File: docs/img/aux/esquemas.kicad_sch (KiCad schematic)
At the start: 60 parts

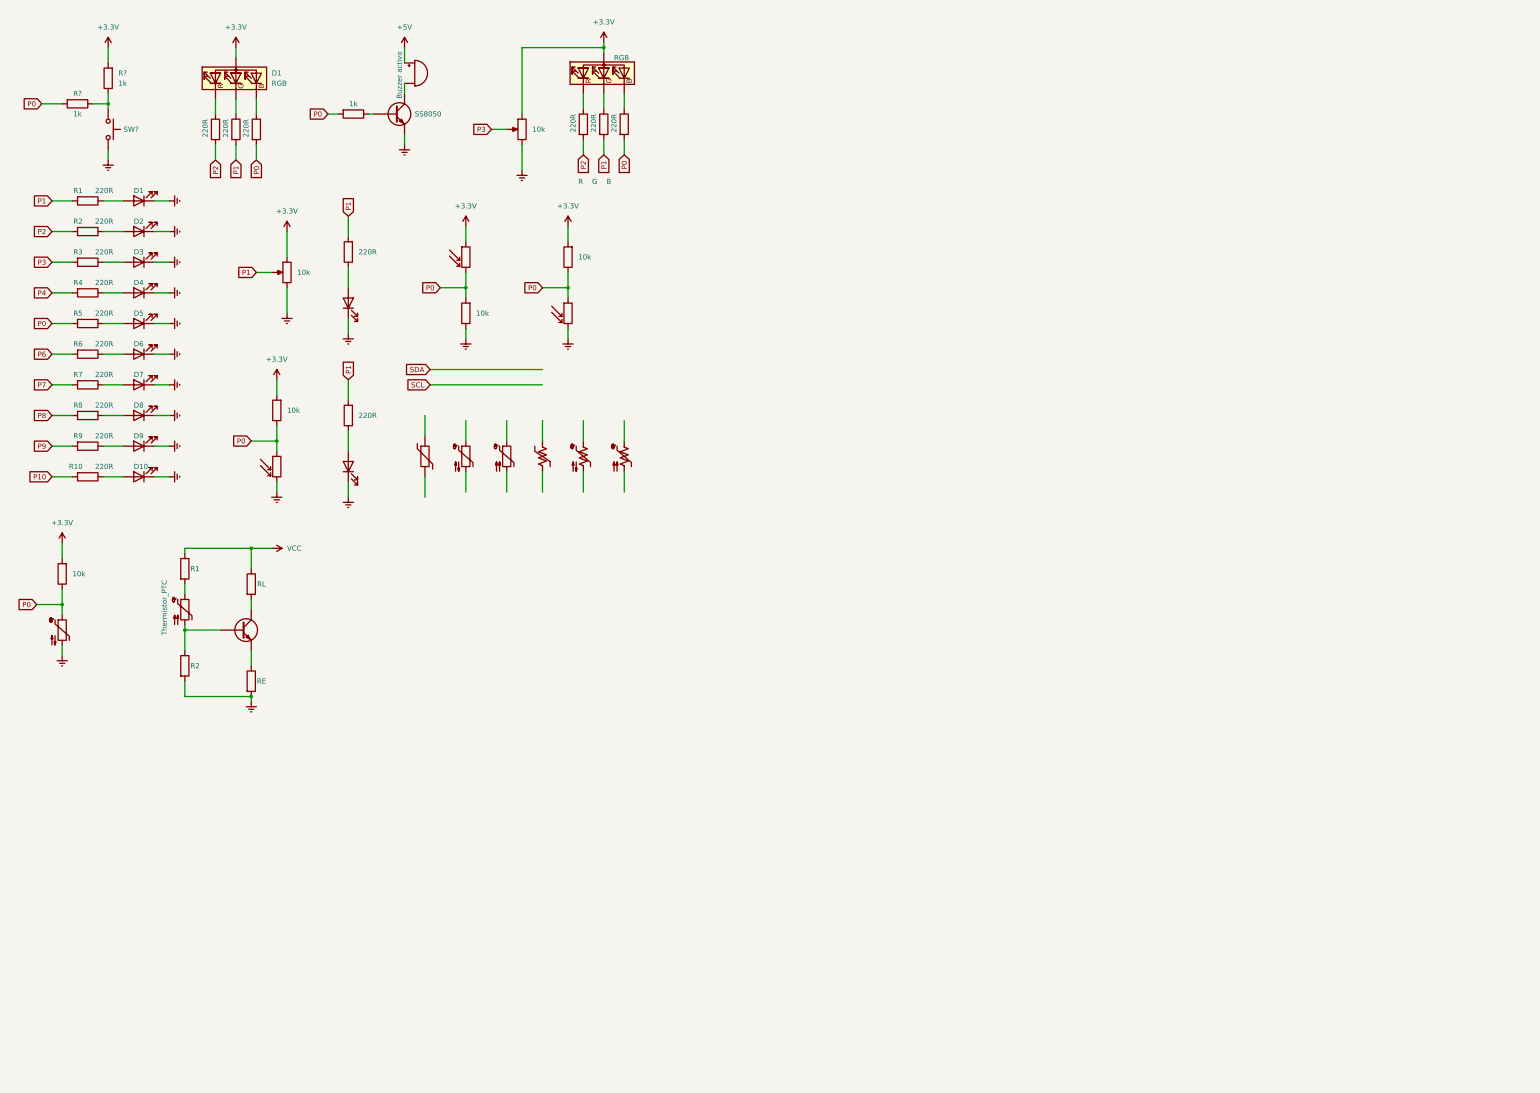
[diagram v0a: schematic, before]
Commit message: actualizar hasta PaP
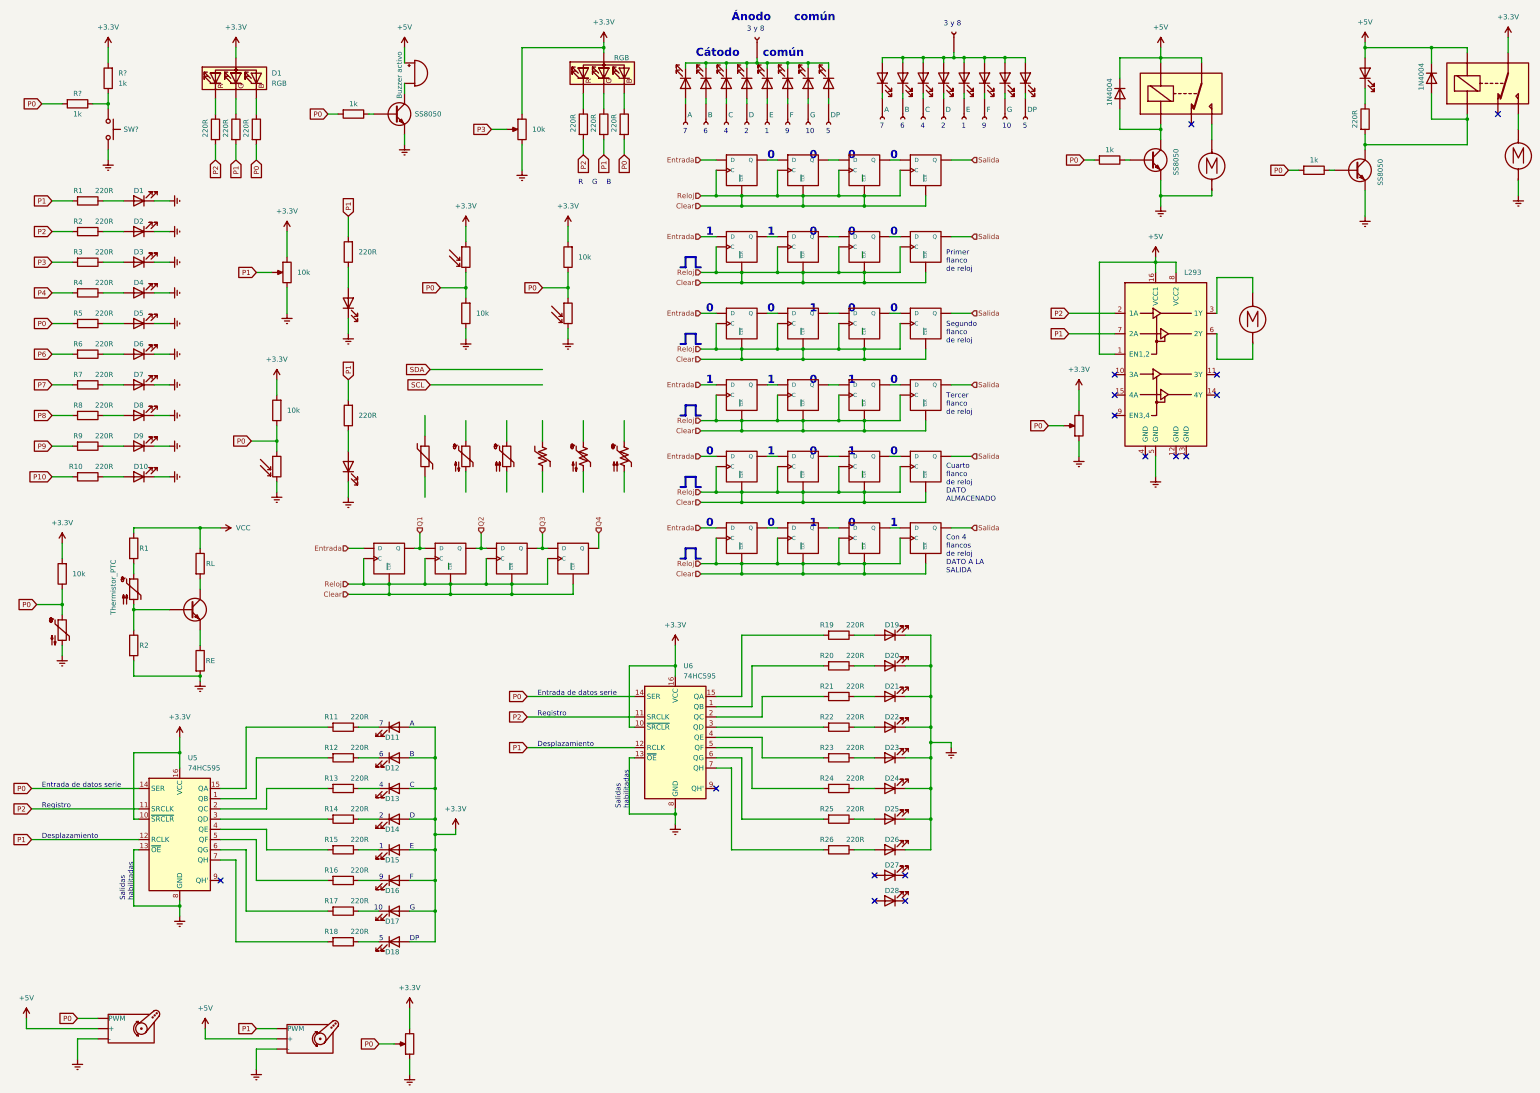
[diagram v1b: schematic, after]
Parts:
- added D11, D12, D13, D14, D15, D16, D17, D18, D19, D20, D21, D22, D23, D24, D25, D26, D27, D28, D? (x17): LED, symbol Device:LED
- added D? (x2): 1N4004, Diode_THT:D_DO-41_SOD81_P10.16mm_Horizontal, symbol Diode:1N4004
- added J? (x2): F, symbol Connector:Conn_01x01_Female
- added J? (x2): C, symbol Connector:Conn_01x01_Female
- added J? (x2): G, symbol Connector:Conn_01x01_Female
- added J? (x2): DP, symbol Connector:Conn_01x01_Female
- added J? (x2): A, symbol Connector:Conn_01x01_Female
- added J? (x2): B, symbol Connector:Conn_01x01_Female
- added J? (x2): D, symbol Connector:Conn_01x01_Female
- added J? (x2): Conn_01x01_Female, symbol Connector:Conn_01x01_Female
- added J? (x2): E, symbol Connector:Conn_01x01_Female
- added K? (x2): FINDER-32.21-x000, Relay_THT:Relay_SPDT_Finder_32.21-x000, symbol Relay:FINDER-32.21-x000
- added M? (x3): Motor_DC, symbol Motor:Motor_DC
- added M? (x2): Motor_Servo, symbol Motor:Motor_Servo
- added Q? (x2): SS8050, Package_TO_SOT_THT:TO-92_Inline, symbol Transistor_BJT:2N3904
- added R11, R12, R13, R14, R15, R16, R17, R18, R19, R20, R21, R22, R23, R24, R25, R26, R?: 220R, symbol Device:R
- added R? (x2): 1k, symbol Device:R
- added RV? (x2): R_Potentiometer, symbol Device:R_Potentiometer
- added U1, U2, U3, U4, U? (x24): 74LVC1G175, symbol 74xGxx:74LVC1G175
- added U5, U6: 74HC595, symbol 74xx:74HC595
- added U?: L293, Package_DIP:DIP-16_W7.62mm, symbol Driver_Motor:L293
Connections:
- net +3.3V: now also D11.2 (A), D12.2 (A), D13.2 (A), D14.2 (A), D15.2 (A), D16.2 (A), D17.2 (A), D18.2 (A), K?.11, RV?.3, RV?.3, U5.10 (~{SRCLR}), U5.16 (VCC), U6.10 (~{SRCLR}), U6.16 (VCC)
- net +5V: now also D?.1 (K), D?.1 (K), D?.2 (A), K?.11, K?.A2, K?.A2, M?.2 (+), M?.2 (+), U?.1 (EN1,2), U?.16 (VCC1), U?.8 (VCC2)
- net GNDREF: now also M?.2 (-), M?.2 (-), Q?.1 (E), Q?.1 (E), RV?.1, RV?.1, U?.5 (GND)
- net P0: now also M?.1 (PWM), R?.2, R?.2, RV?.2, RV?.2, U5.14 (SER), U6.14 (SER)
- net P1: now also M?.1 (PWM), U5.12 (RCLK), U6.12 (RCLK), U?.7 (2A)
- net P2: now also U5.11 (SRCLK), U6.11 (SRCLK), U?.2 (1A)
- net VCC: now also U1.5 (VCC), U2.5 (VCC), U3.5 (VCC), U4.5 (VCC), U?.5 (VCC), U?.5 (VCC), U?.5 (VCC), U?.5 (VCC), U?.5 (VCC), U?.5 (VCC), U?.5 (VCC), U?.5 (VCC), U?.5 (VCC), U?.5 (VCC), U?.5 (VCC), U?.5 (VCC), U?.5 (VCC), U?.5 (VCC), U?.5 (VCC), U?.5 (VCC), U?.5 (VCC), U?.5 (VCC), U?.5 (VCC), U?.5 (VCC), U?.5 (VCC), U?.5 (VCC), U?.5 (VCC), U?.5 (VCC)
- new net: D?.1 (K), J?.1 (Pin_1) (x8)
- new net: D?.2 (A), D?.2 (A), D?.2 (A), D?.2 (A), D?.2 (A), D?.2 (A), D?.2 (A), D?.2 (A), J?.1 (Pin_1)
- new net: R12.2, U5.1 (QB)
- new net: R11.2, U5.15 (QA)
- new net: R13.2, U5.2 (QC)
- new net: R14.2, U5.3 (QD)
- new net: R15.2, U5.4 (QE)
- new net: R16.2, U5.5 (QF)
- new net: R17.2, U5.6 (QG)
- new net: R18.2, U5.7 (QH)
- new net: D?.2 (A), K?.A1, Q?.3 (C), R?.2
- new net: D13.1 (K), R13.1
- new net: U?.3 (D), U?.4 (Q) (x15)
- new net: D19.2 (A), R19.1
- new net: D16.1 (K), R16.1
- new net: D?.2 (A), J?.1 (Pin_1) (x8)
- new net: Q?.2 (B), R?.1 (x2)
- new net: D17.1 (K), R17.1
- new net: D12.1 (K), R12.1
- new net: D14.1 (K), R14.1
- new net: D26.2 (A), R26.1
- new net: R26.2, U6.7 (QH)
- new net: D24.2 (A), R24.1
- new net: R24.2, U6.5 (QF)
- new net: D21.2 (A), R21.1
- new net: U3.4 (Q), U4.3 (D)
- new net: K?.14, M?.1 (+) (x2)
- new net: D23.2 (A), R23.1
- new net: R23.2, U6.4 (QE)
- new net: D25.2 (A), R25.1
- new net: R21.2, U6.2 (QC)
- new net: D?.1 (K), R?.1
- new net: D11.1 (K), R11.1
- new net: D22.2 (A), R22.1
- new net: R22.2, U6.3 (QD)
- new net: D?.1 (K), D?.1 (K), D?.1 (K), D?.1 (K), D?.1 (K), D?.1 (K), D?.1 (K), D?.1 (K), J?.1 (Pin_1)
- new net: R20.2, U6.1 (QB)
- new net: R19.2, U6.15 (QA)
- new net: R25.2, U6.6 (QG)
- new net: D?.2 (A), K?.A1, Q?.3 (C)
- new net: M?.1 (+), U?.3 (1Y)
- new net: M?.2 (-), U?.6 (2Y)
- new net: D15.1 (K), R15.1
- new net: U1.4 (Q), U2.3 (D)
- new net: U2.4 (Q), U3.3 (D)
- new net: D18.1 (K), R18.1
- new net: D20.2 (A), R20.1
- new net Clear: U1.1 (C), U1.6 (~{CLR}), U2.1 (C), U2.6 (~{CLR}), U3.1 (C), U3.6 (~{CLR}), U4.1 (C), U4.6 (~{CLR}), U?.1 (C), U?.1 (C), U?.1 (C), U?.1 (C), U?.1 (C), U?.1 (C), U?.1 (C), U?.1 (C), U?.1 (C), U?.1 (C), U?.1 (C), U?.1 (C), U?.1 (C), U?.1 (C), U?.1 (C), U?.1 (C), U?.1 (C), U?.1 (C), U?.1 (C), U?.1 (C), U?.1 (C), U?.1 (C), U?.1 (C), U?.1 (C), U?.6 (~{CLR}), U?.6 (~{CLR}), U?.6 (~{CLR}), U?.6 (~{CLR}), U?.6 (~{CLR}), U?.6 (~{CLR}), U?.6 (~{CLR}), U?.6 (~{CLR}), U?.6 (~{CLR}), U?.6 (~{CLR}), U?.6 (~{CLR}), U?.6 (~{CLR}), U?.6 (~{CLR}), U?.6 (~{CLR}), U?.6 (~{CLR}), U?.6 (~{CLR}), U?.6 (~{CLR}), U?.6 (~{CLR}), U?.6 (~{CLR}), U?.6 (~{CLR}), U?.6 (~{CLR}), U?.6 (~{CLR}), U?.6 (~{CLR}), U?.6 (~{CLR})
- new net Earth: D19.1 (K), D20.1 (K), D21.1 (K), D22.1 (K), D23.1 (K), D24.1 (K), D25.1 (K), D26.1 (K), M?.3 (-), M?.3 (-), U5.13 (~{OE}), U5.8 (GND), U6.13 (~{OE}), U6.8 (GND)
- new net Entrada: U1.3 (D), U?.3 (D), U?.3 (D), U?.3 (D), U?.3 (D), U?.3 (D), U?.3 (D)
- new net GND: U1.2 (GND), U2.2 (GND), U3.2 (GND), U4.2 (GND), U?.2 (GND), U?.2 (GND), U?.2 (GND), U?.2 (GND), U?.2 (GND), U?.2 (GND), U?.2 (GND), U?.2 (GND), U?.2 (GND), U?.2 (GND), U?.2 (GND), U?.2 (GND), U?.2 (GND), U?.2 (GND), U?.2 (GND), U?.2 (GND), U?.2 (GND), U?.2 (GND), U?.2 (GND), U?.2 (GND), U?.2 (GND), U?.2 (GND), U?.2 (GND), U?.2 (GND)
- new net Q1: U?.3 (D), U?.4 (Q)
- new net Q2: U?.3 (D), U?.4 (Q)
- new net Q3: U?.3 (D), U?.4 (Q)
- new net Q4: U?.4 (Q)
- new net Salida: U4.4 (Q), U?.4 (Q), U?.4 (Q), U?.4 (Q), U?.4 (Q), U?.4 (Q)
- no-connect marks 0 -> 16
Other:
- note added: "0"
- note added: "0 0 0 0"
- note added: "0 1 0 0"
- note added: "0 1 0 1"
- note added: "1"
- note added: "1 0 0 0"
- note added: "1 0 1 0"
- note added: "10"
- note added: "2"
- note added: "3 y 8"
- note added: "4"
- note added: "5"
- note added: "6"
- note added: "7"
- note added: "9"
- note added: "A"
- note added: "B"
- note added: "C"
- note added: "Con 4 flancos de reloj DATO A LA SALIDA"
- note added: "Cuarto flanco de reloj DATO ALMACENADO"
- note added: "Cátodo común"
- note added: "D"
- note added: "DP"
- note added: "Desplazamiento"
- note added: "E"
- note added: "Entrada de datos serie"
- note added: "F"
- note added: "G"
- note added: "Primer flanco de reloj"
- note added: "Registro"
- note added: "Salidas habilitadas"
- note added: "Segundo flanco de reloj"
- note added: "Tercer flanco de reloj"
- note added: "Ánodo común"
- moved on the sheet: R1, R2, RE, RL
